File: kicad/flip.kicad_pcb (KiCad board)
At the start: 2 copper layers, 95 x 62 mm, 20 parts, among them J1 CHANNEL, J2 COILS, J3 IDC1, J4 GROUND, J5 HAL_TEST, Q1 Q_NPN_BEC, Q2 Q_NPN_BEC, Q3 Q_NPN_BEC, Q4 Q_NPN_BEC

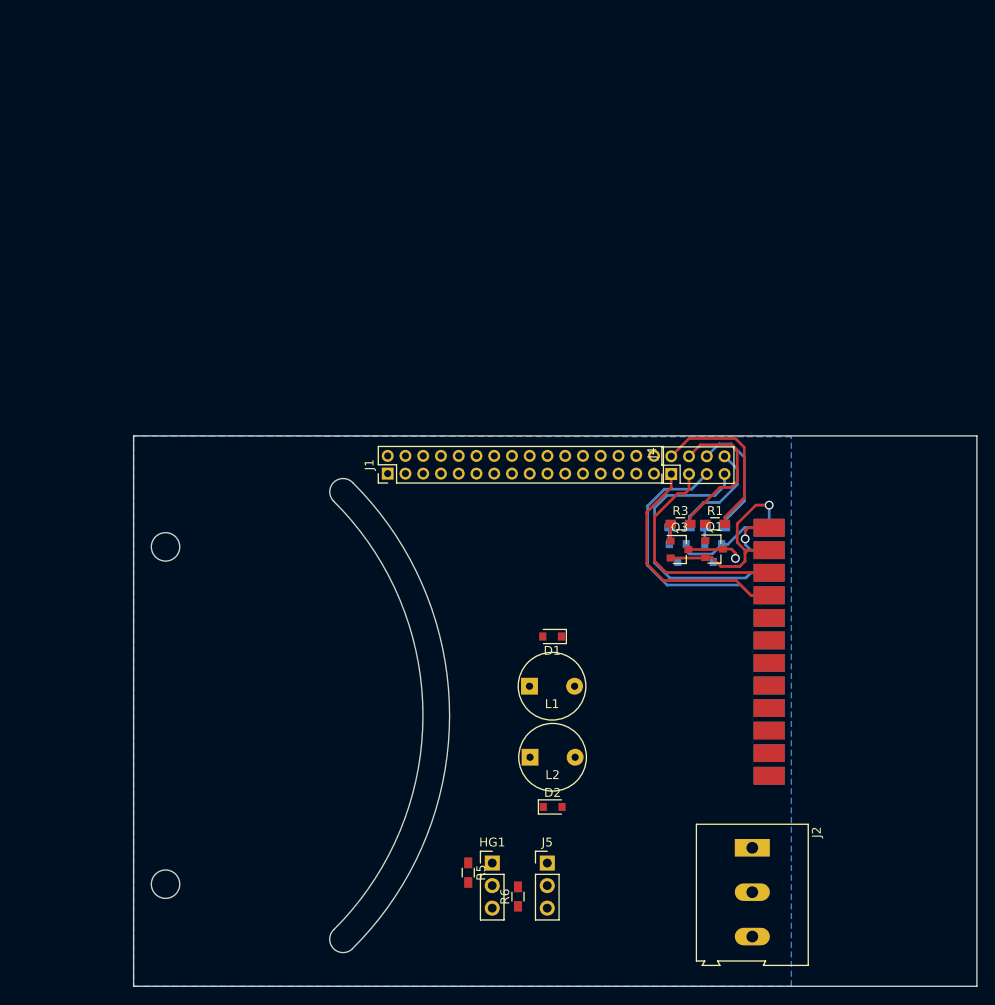
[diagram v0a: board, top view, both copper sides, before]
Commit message: new PCB ready
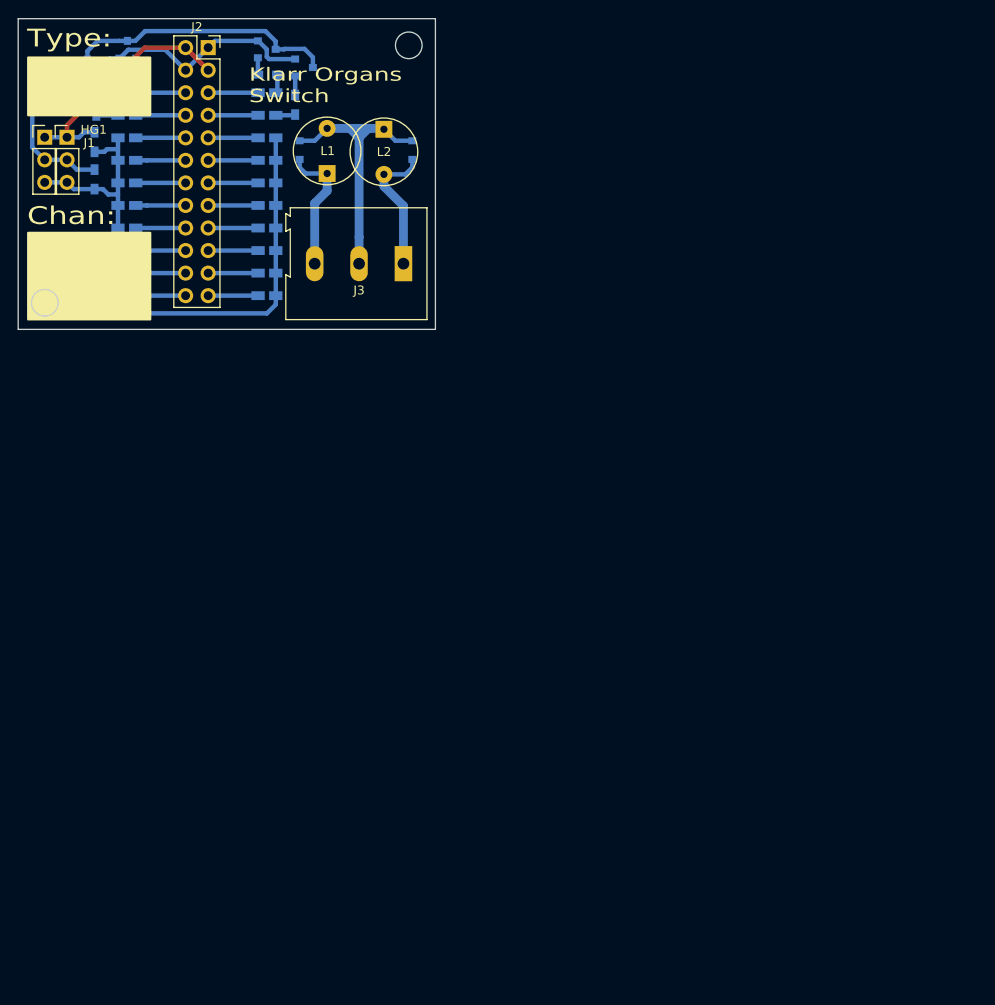
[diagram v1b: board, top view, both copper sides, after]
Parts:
- removed J4: GROUND, Pin_Headers:Pin_Header_Straight_2x04_Pitch2.00mm
- removed J5: HAL_TEST, Pin_Headers:Pin_Header_Straight_1x03_Pitch2.54mm
- added C0: J1, #MOJABIBLIOTEKA:Jumper_SMD, B.Cu at (159.0, 58.4)
- added C1: J2, #MOJABIBLIOTEKA:Jumper_SMD, B.Cu at (159.0, 61.0)
- added C10: J11, #MOJABIBLIOTEKA:Jumper_SMD, B.Cu at (143.2, 71.1)
- added C11: J12, #MOJABIBLIOTEKA:Jumper_SMD, B.Cu at (143.2, 68.6)
- added C12: J13, #MOJABIBLIOTEKA:Jumper_SMD, B.Cu at (143.2, 66.0)
- added C13: J14, #MOJABIBLIOTEKA:Jumper_SMD, B.Cu at (143.2, 63.5)
- added C14: J15, #MOJABIBLIOTEKA:Jumper_SMD, B.Cu at (143.2, 61.0)
- added C15: J16, #MOJABIBLIOTEKA:Jumper_SMD, B.Cu at (143.2, 58.4)
- added C2: J3, #MOJABIBLIOTEKA:Jumper_SMD, B.Cu at (159.0, 63.5)
- added C3: J4, #MOJABIBLIOTEKA:Jumper_SMD, B.Cu at (159.0, 66.0)
- added C4: J5, #MOJABIBLIOTEKA:Jumper_SMD, B.Cu at (159.0, 68.6)
- added C5: J6, #MOJABIBLIOTEKA:Jumper_SMD, B.Cu at (159.0, 71.1)
- added C6: J7, #MOJABIBLIOTEKA:Jumper_SMD, B.Cu at (159.0, 73.7)
- added C7: J8, #MOJABIBLIOTEKA:Jumper_SMD, B.Cu at (159.0, 76.2)
- added C8: J9, #MOJABIBLIOTEKA:Jumper_SMD, B.Cu at (143.2, 76.2)
- added C9: J10, #MOJABIBLIOTEKA:Jumper_SMD, B.Cu at (143.2, 73.7)
- added G0: G4, #MOJABIBLIOTEKA:Jumper_SMD, B.Cu at (159.0, 53.3)
- added G1: G3, #MOJABIBLIOTEKA:Jumper_SMD, B.Cu at (159.0, 55.9)
- added G2: G1, #MOJABIBLIOTEKA:Jumper_SMD, B.Cu at (143.2, 55.9)
- added G3: G2, #MOJABIBLIOTEKA:Jumper_SMD, B.Cu at (143.2, 53.3)
- D1, D2, Q1, Q3, R1: moved to B.Cu
- J1: value CHANNEL -> HAL_TEST; footprint Pin_Headers:Pin_Header_Straight_2x16_Pitch2.00mm -> Pin_Headers:Pin_Header_Straight_1x03_Pitch2.54mm
- J2: value COILS -> IDC1; footprint Connectors_Terminal_Blocks:TerminalBlock_Altech_AK300-3_P5.00mm -> Socket_Strips:Socket_Strip_Straight_2x12_Pitch2.54mm
- J3: value IDC1 -> COILS; footprint #MOJABIBLIOTEKA:IDC_edge -> Connectors_Terminal_Blocks:TerminalBlock_Altech_AK300-3_P5.00mm; moved to F.Cu
- R2: value 3k3 -> [10k]
- R3: value 3k3 -> [10k]; moved to B.Cu
- R5, R6: value [10k] -> 3k3; moved to B.Cu
- moved J2 109.0 mm to (152.4, 48.3), turned to 0 degrees
- moved R5 97.8 mm to (143.3, 51.2), turned to 180 degrees
- moved R6 96.8 mm to (159.1, 51.3), turned to 0 degrees
- moved HG1 94.8 mm to (136.5, 58.4)
- moved Q1 89.0 mm to (138.8, 50.6), turned to 90 degrees
- moved R1 84.1 mm to (139.8, 54.8), turned to 270 degrees
- moved Q3 83.9 mm to (143.3, 48.5), turned to 90 degrees
- moved R2 82.3 mm to (139.6, 58.9), turned to 270 degrees
- moved R3 76.6 mm to (139.6, 63.1), turned to 90 degrees
- moved D2 75.7 mm to (175.4, 59.8), turned to 270 degrees
- moved Q4 73.2 mm to (159.0, 48.5), turned to 0 degrees
- moved Q2 71.5 mm to (163.2, 50.5), turned to 0 degrees
- moved L2 70.8 mm to (172.2, 60.0), turned to 270 degrees
- moved L1 65.4 mm to (165.8, 59.9), turned to 90 degrees
- moved R4 64.3 mm to (162.2, 54.7), turned to 270 degrees
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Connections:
- J1 pad 1: CH01 -> VCC
- J1 pad 2: DIGITAL -> SW_GND
- J1 pad 3: CH02 -> DIGITAL
- J2 pad 1: Net-(D2-Pad2) -> GND
- J2 pad 2: Net-(D1-Pad1) -> VCC
- J2 pad 3: Net-(D1-Pad2) -> VCC
- J3 pad 1: GND -> Net-(D2-Pad2)
- J3 pad 2: VCC -> Net-(D1-Pad1)
- J3 pad 3: VCC -> Net-(D1-Pad2)
- R2 pad 1: Net-(Q2-Pad1) -> VCC
- R2 pad 2: SW_GND2 -> DIGITAL
- R3 pad 1: Net-(Q3-Pad1) -> DIGITAL
- R3 pad 2: SW_GND1 -> SW_GND
- R4 pad 1: Net-(Q4-Pad1) -> Net-(Q2-Pad1)
- R4 pad 2: SW_GND3 -> SW_GND2
- R5 pad 1: VCC -> Net-(Q3-Pad1)
- R5 pad 2: DIGITAL -> SW_GND1
- R6 pad 1: DIGITAL -> Net-(Q4-Pad1)
- R6 pad 2: SW_GND -> SW_GND3
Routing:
- net DIGITAL: track 0.00 -> 67.8 mm
- net SW_GND: track 6.45 -> 51.9 mm, vias 1 -> 0
- net Net-(D1-Pad1): track 0.00 -> 32.3 mm
- net GND0: track 30.3 -> 5.62 mm
- net GND1: track 30.0 -> 5.62 mm
- net GND2: track 26.5 -> 5.62 mm
- net VCC: track 7.35 -> 27.8 mm, vias 1 -> 0
- net GND3: track 25.3 -> 5.62 mm
- net SW_GND0: track 19.0 -> 2.45 mm
- net Net-(D2-Pad2): track 0.00 -> 15.4 mm
- net SW_GND1: track 17.4 -> 2.16 mm
- net Net-(D1-Pad2): track 0.00 -> 15.0 mm
- net SW_GND2: track 14.2 -> 2.21 mm
- net SW_GND3: track 11.9 -> 2.11 mm
- net GND: track 38.1 -> 29.3 mm, vias 1 -> 0
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- removed copper zone on B.Cu, net SW_GND
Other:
- board size 95 x 62 mm -> 47 x 35 mm
- net class Default: clearance 0.25 -> 0.2; trace_width 0.3 -> 0.25; via_dia 1 -> 0.6; via_drill 0.7 -> 0.4
- net class PWR added: clearance 0.7, trace_width 1, via_dia 1, via_drill 0.7
- net class Power removed
- net class SIG added: clearance 0.3, trace_width 0.5, via_dia 0.7, via_drill 0.4
- rule pad_to_mask_clearance: 0.2 -> 0
- rule trace_clearance: 0.25 -> 0.2
- board text added: "Chan:"
- board text added: "Klarr Organs Switch"
- board text added: "Type:"
